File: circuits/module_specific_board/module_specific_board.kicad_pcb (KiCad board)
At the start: 2 copper layers, 26.7 x 91.4 mm, 18 parts, among them J1 Pot, J2 Pot, J3 Pot, J4 Pot, P1 CONN_01X08, P10 CONN_01X01, P2 CONN_01X08, P3 CONN_01X08, P4 CONN_01X08, P5 CONN_01X08, P6 CONN_01X02, P7 CONN_01X04, P8 CONN_01X02, P9 CONN_01X01

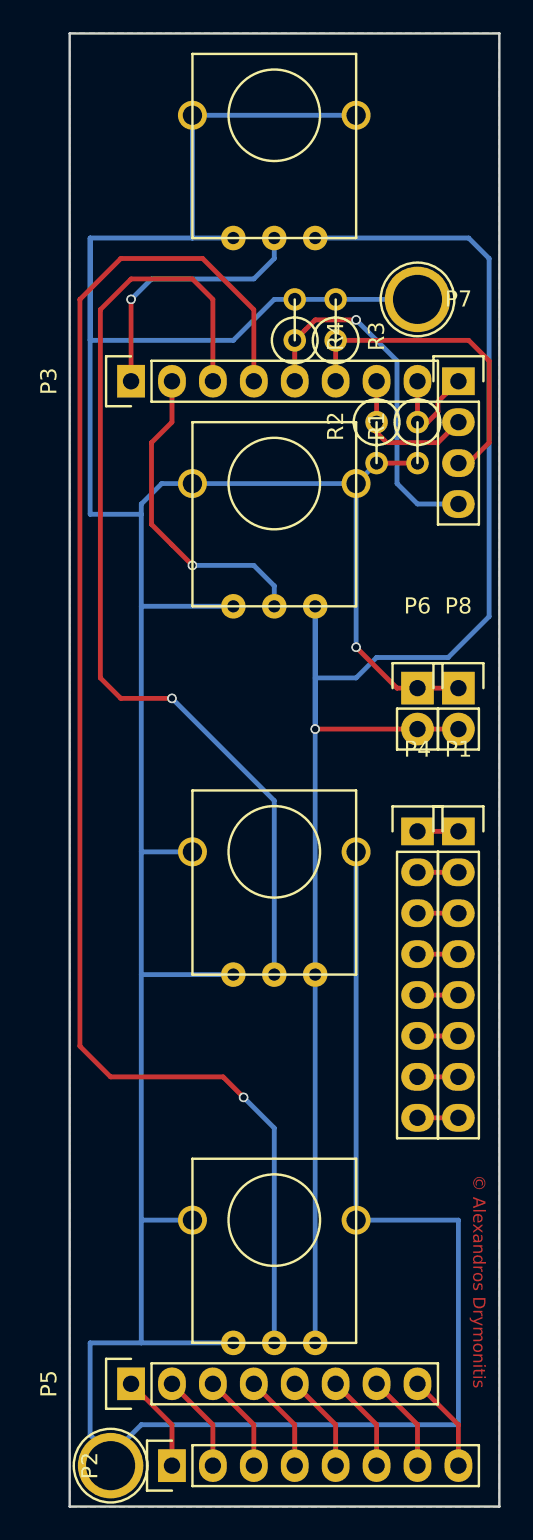
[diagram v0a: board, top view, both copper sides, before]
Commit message: Update circuits
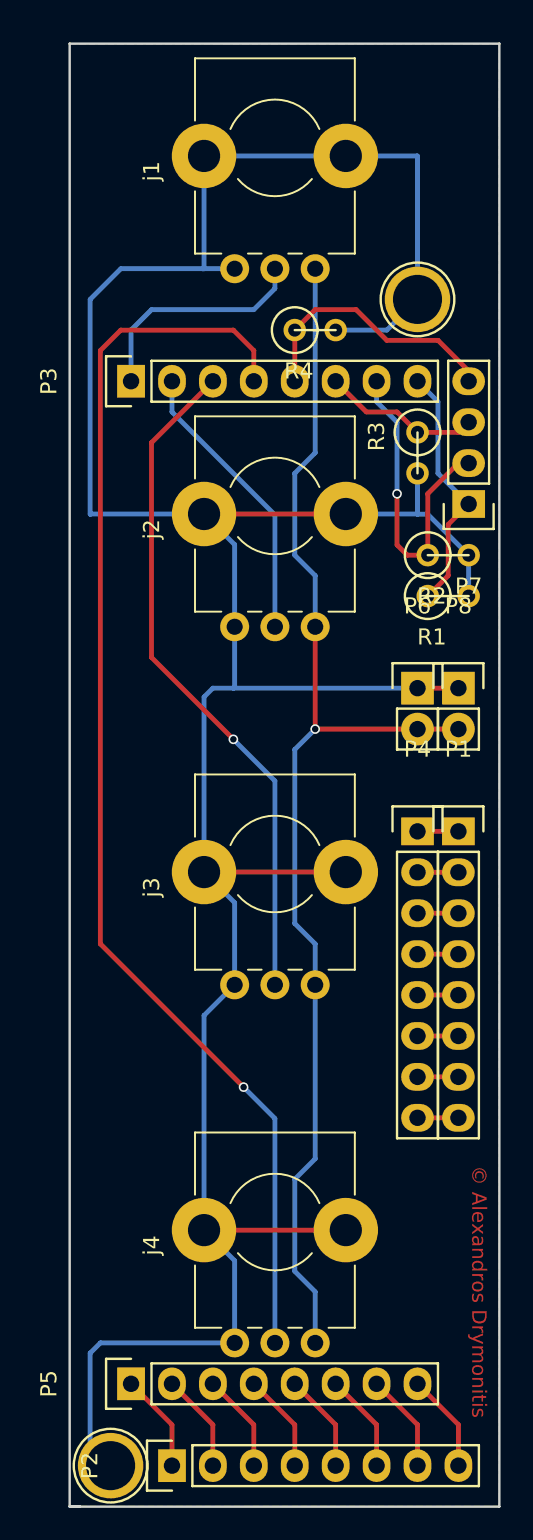
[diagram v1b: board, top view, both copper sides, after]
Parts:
- removed J1, J2, J3, J4: Pot, pot:Pot
- added j1: ALPSpot097, Potentiometers:Potentiometer_Alps_RK09K_Horizontal, F.Cu at (138.4, 64.1)
- added j2: ALPSpot097, Potentiometers:Potentiometer_Alps_RK09K_Horizontal, F.Cu at (138.4, 86.4)
- added j3: ALPSpot097, Potentiometers:Potentiometer_Alps_RK09K_Horizontal, F.Cu at (138.4, 108.6)
- added j4: ALPSpot097, Potentiometers:Potentiometer_Alps_RK09K_Horizontal, F.Cu at (138.4, 130.8)
- moved R1 9.71 mm to (146.7, 84.5), turned to 0 degrees
- moved R3 9.69 mm to (144.8, 75.6), turned to 270 degrees
- moved R2 8.28 mm to (146.7, 81.9), turned to 0 degrees
- moved P7 7.65 mm to (148.0, 78.7), turned to 180 degrees
- moved R4 1.42 mm to (138.4, 67.9), turned to 0 degrees
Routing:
- net GND: track 262.3 -> 193.5 mm, vias 1 -> 0
- net VCC: track 108.1 -> 78.7 mm
- net /POT3: track 61.0 -> 42.2 mm
- net /POT4: track 91.5 -> 78.6 mm
- net /MUX7: track 9.04 -> 20.0 mm, vias 0 -> 1
- net /MUX6: track 20.1 -> 9.83 mm
- net /MUX8: track 6.50 -> 15.7 mm
- net /MUX5: track 22.4 -> 16.7 mm, vias 1 -> 0
- net /POT2: track 19.9 -> 17.9 mm, vias 1 -> 0
- net /POT1: track 16.3 -> 14.4 mm, vias 1 -> 0
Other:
- board size 26.7 x 91.4 mm -> 26.7 x 90.8 mm
